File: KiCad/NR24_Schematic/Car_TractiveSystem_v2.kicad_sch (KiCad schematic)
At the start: 15 parts, among them J1 M_con, J2 F_con, K2 Key Switch Relay, M1 Zero_7R_Motor, SW3 100V E-stop (Right), SW4 100V E-stop (Left), SW7 TI power switch, SW8 GLVMS, U1 Sevcon_Gen4_Size6, U2 Throttle, U7 Brake (AiM Pressure Sensor)

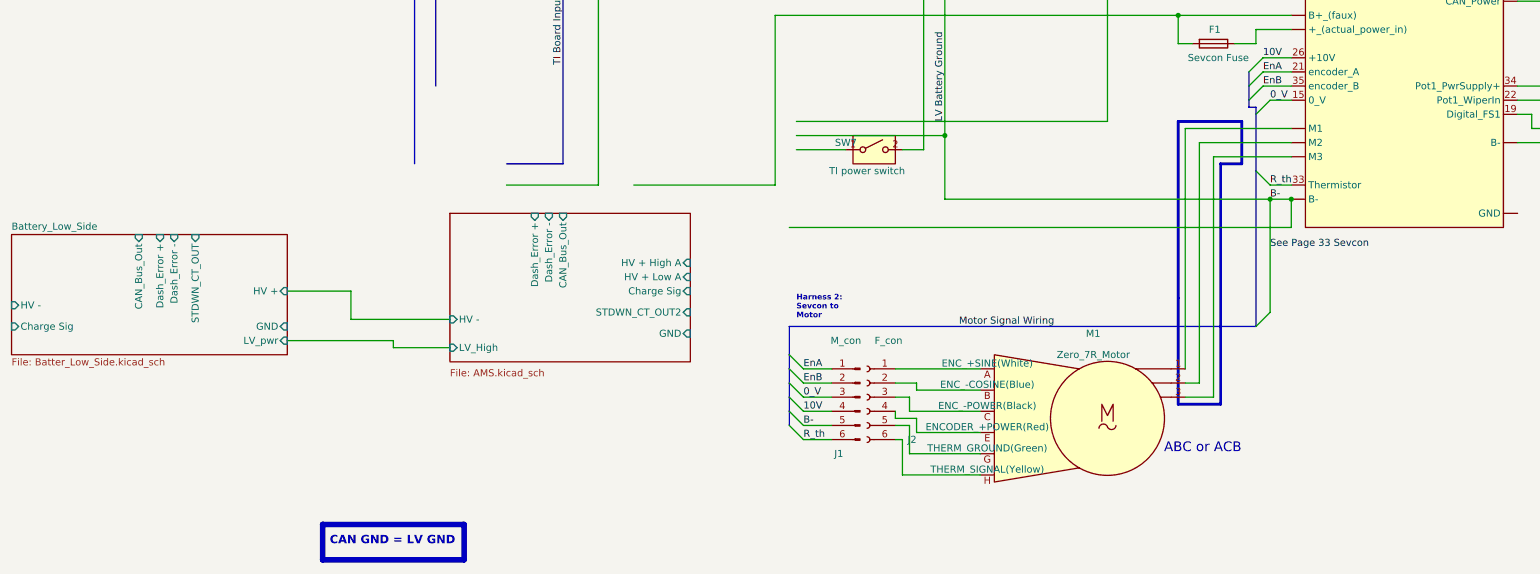
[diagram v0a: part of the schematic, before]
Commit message: update
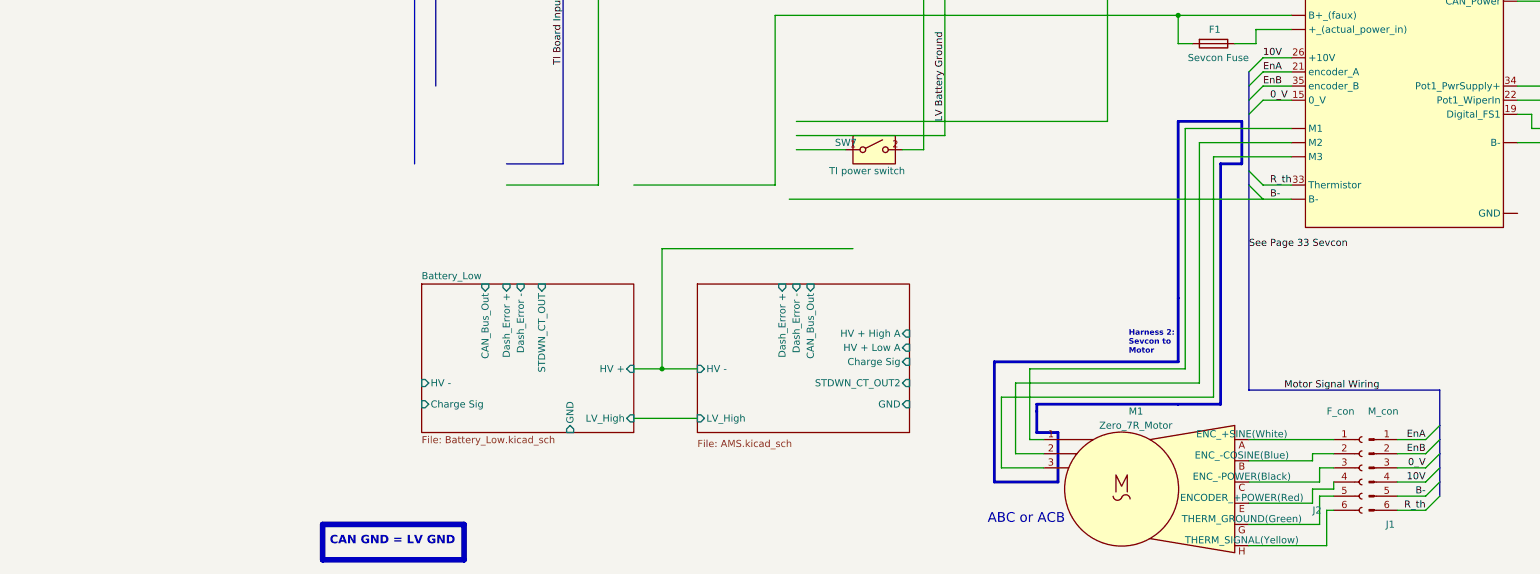
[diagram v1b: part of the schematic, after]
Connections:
- net B-: no longer BTaux1.2 (-), LA6.1 (-)
- new net LV Battery Ground: BTaux1.2 (-), LA6.1 (-)
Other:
- sheet Battery_Low_Side renamed Battery_Low
- sheet Battery_Low: file Batter_Low_Side.kicad_sch -> Battery_Low.kicad_sch
- sheet Battery_Low ports: added LV_High; removed LV_pwr
- moved on the sheet: J1, J2, M1
